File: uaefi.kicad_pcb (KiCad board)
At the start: 4 copper layers, 155 x 148 mm, 127 parts, among them J6 Conn_01x06, J7 Conn_01x05_Male, J8 USB_B_Mini, J9 USB_C, M1 Module-power_12and5V-0.3, M2 Module-knock-0.2, M3 Module-vr-discrete-0.5, M4 Module-vr-max9924-0.1, M5 Module-wbo-0.5, M6 Module:mega-mcu100/0.3, M7 Module-can-0.1, P3 Pad, P4 Pad, P5 Pad, P6 Pad, P7 Pad, P8 Pad, P9 963356-1, Q10 ISL9V3040D3ST, Q11 ISL9V3040D3ST, Q12 ISL9V3040D3ST, Q7 ISL9V3040D3ST, Q8 ISL9V3040D3ST, Q9 ISL9V3040D3ST, U1 TLE9201SG, U10 VNLD5160TR-E, U11 VNLD5160TR-E, U2 TLE9201SG, U3 MPX4/MPXH6400_MAP, U4 MAX31855KASA, U5 JDY-33, U6 VNLD5160TR-E, U7 VNLD5160TR-E, U8 VNLD5160TR-E, U9 VNLD5160TR-E

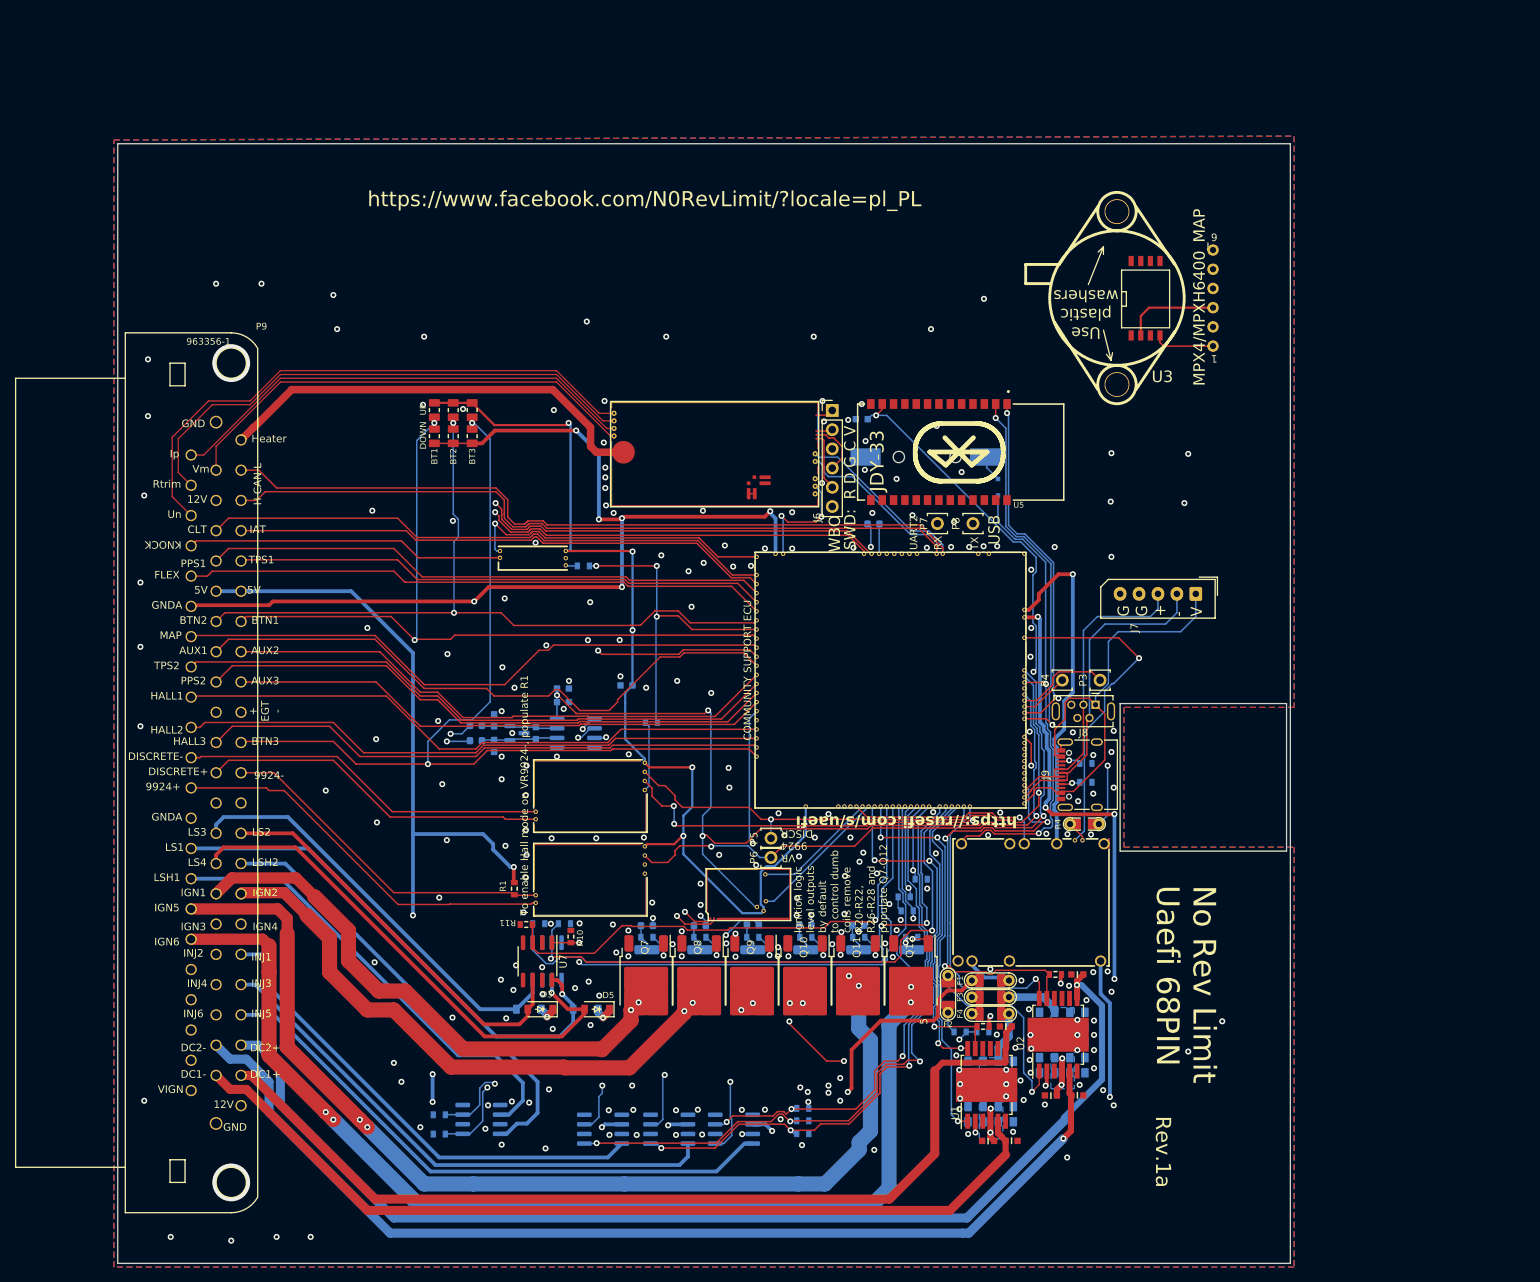
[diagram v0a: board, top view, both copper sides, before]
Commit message: can2, egt, przesyniecie pcb
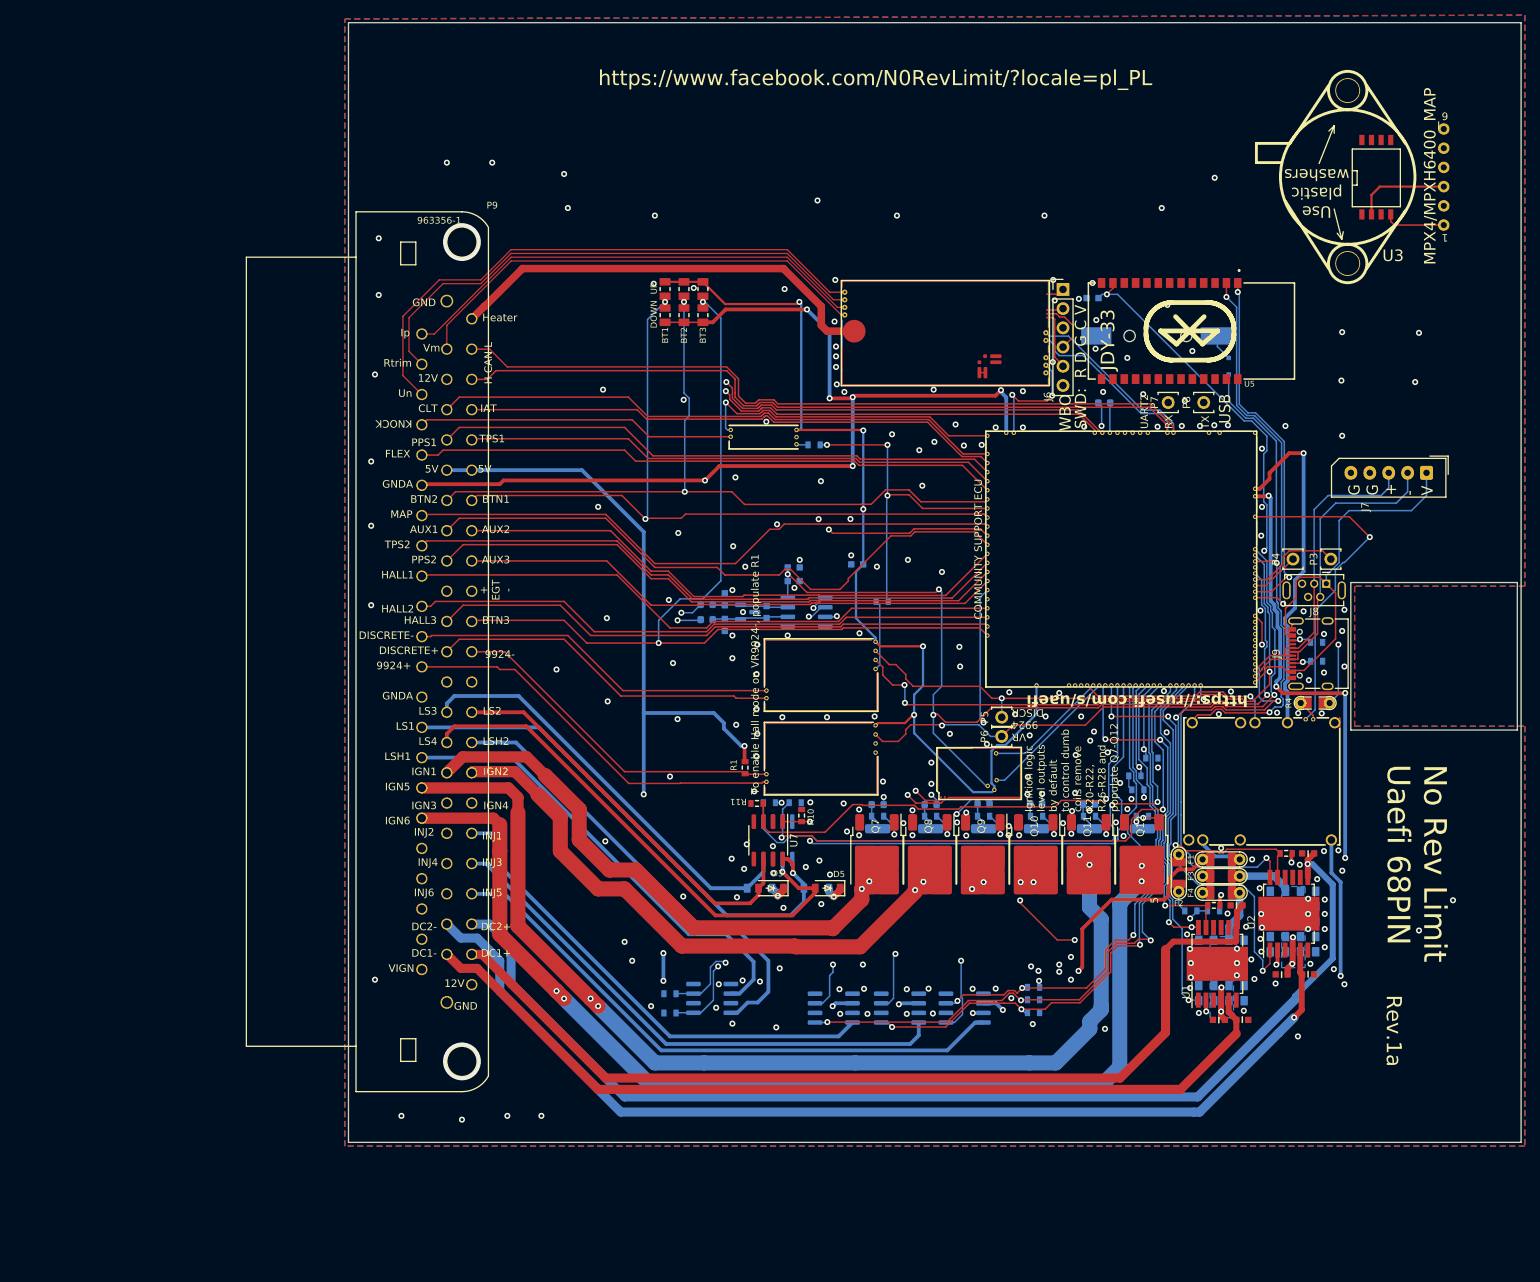
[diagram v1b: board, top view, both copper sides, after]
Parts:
- moved J6 34.4 mm to (144.5, 47.3)
- moved R19 34.4 mm to (134.0, 116.9)
- moved R23 34.4 mm to (141.0, 116.9)
- moved R24 34.4 mm to (148.0, 116.9)
- moved R25 34.4 mm to (155.0, 116.9)
- moved R30 34.4 mm to (156.2, 109.2)
- moved R32 34.4 mm to (154.0, 111.6)
- moved U11 34.4 mm to (131.5, 142.3)
- moved F1 34.4 mm to (165.4, 122.6)
- moved F5 34.4 mm to (127.0, 115.4)
- moved F6 34.4 mm to (120.0, 115.4)
- moved P8 34.4 mm to (163.1, 62.2)
- moved R12 34.4 mm to (105.7, 115.1)
- moved R13 34.4 mm to (109.1, 115.1)
- moved C1 34.4 mm to (163.4, 141.3)
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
